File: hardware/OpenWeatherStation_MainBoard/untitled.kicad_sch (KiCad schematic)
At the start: 46 parts, among them Q1 Q_NMOS_GDS, U5 PM8800A, U6 POE13P-33L

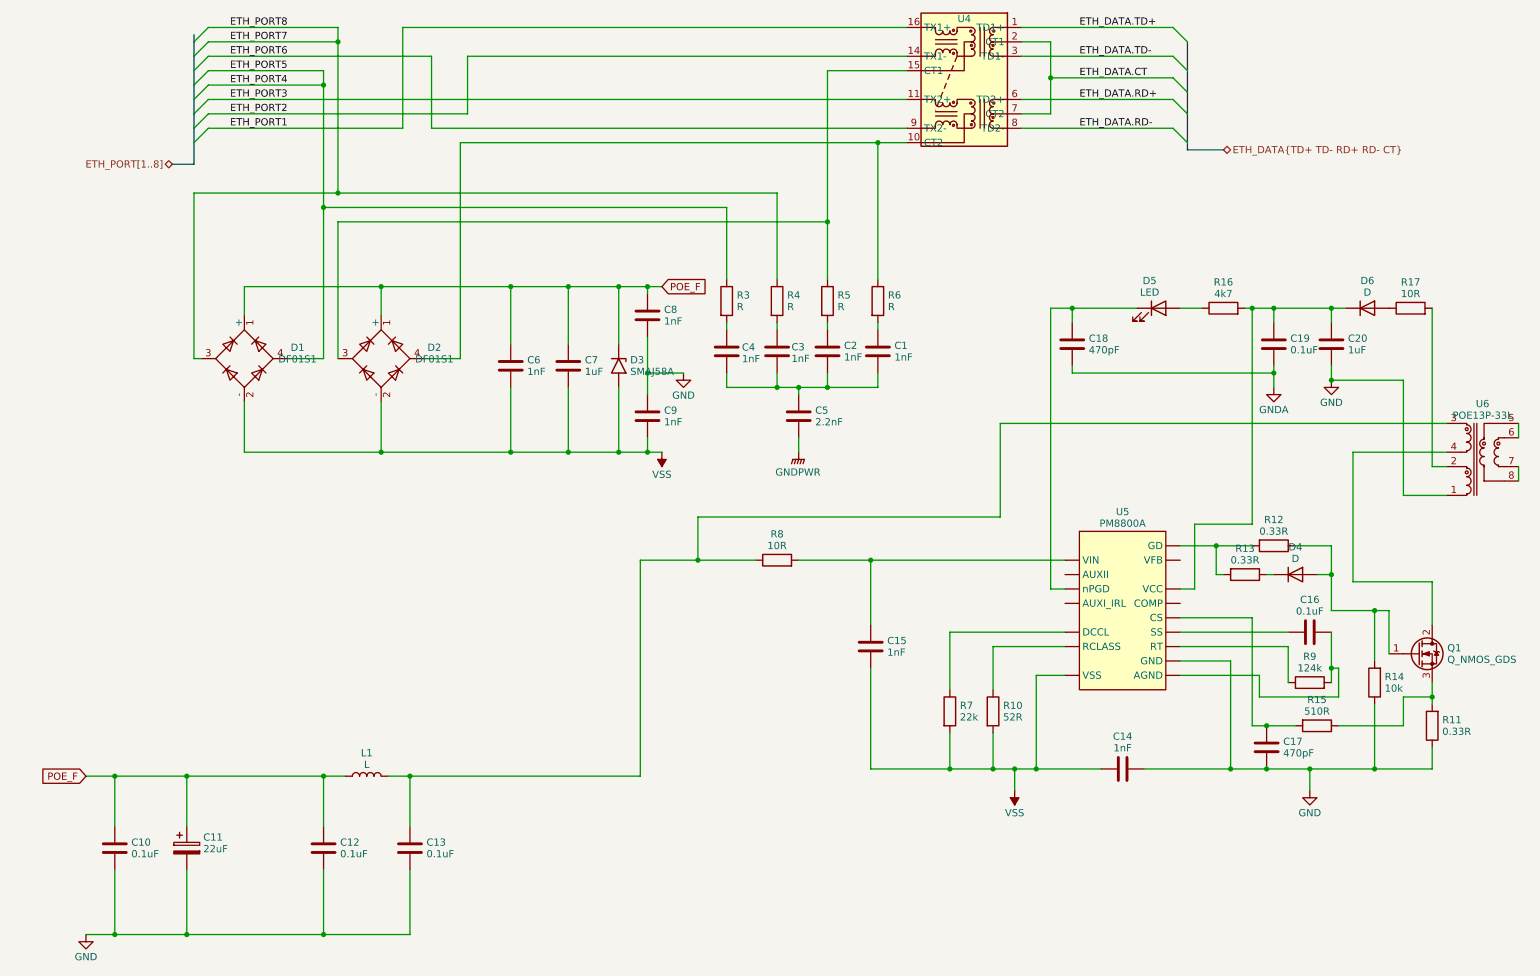
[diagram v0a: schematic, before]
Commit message: poe wip
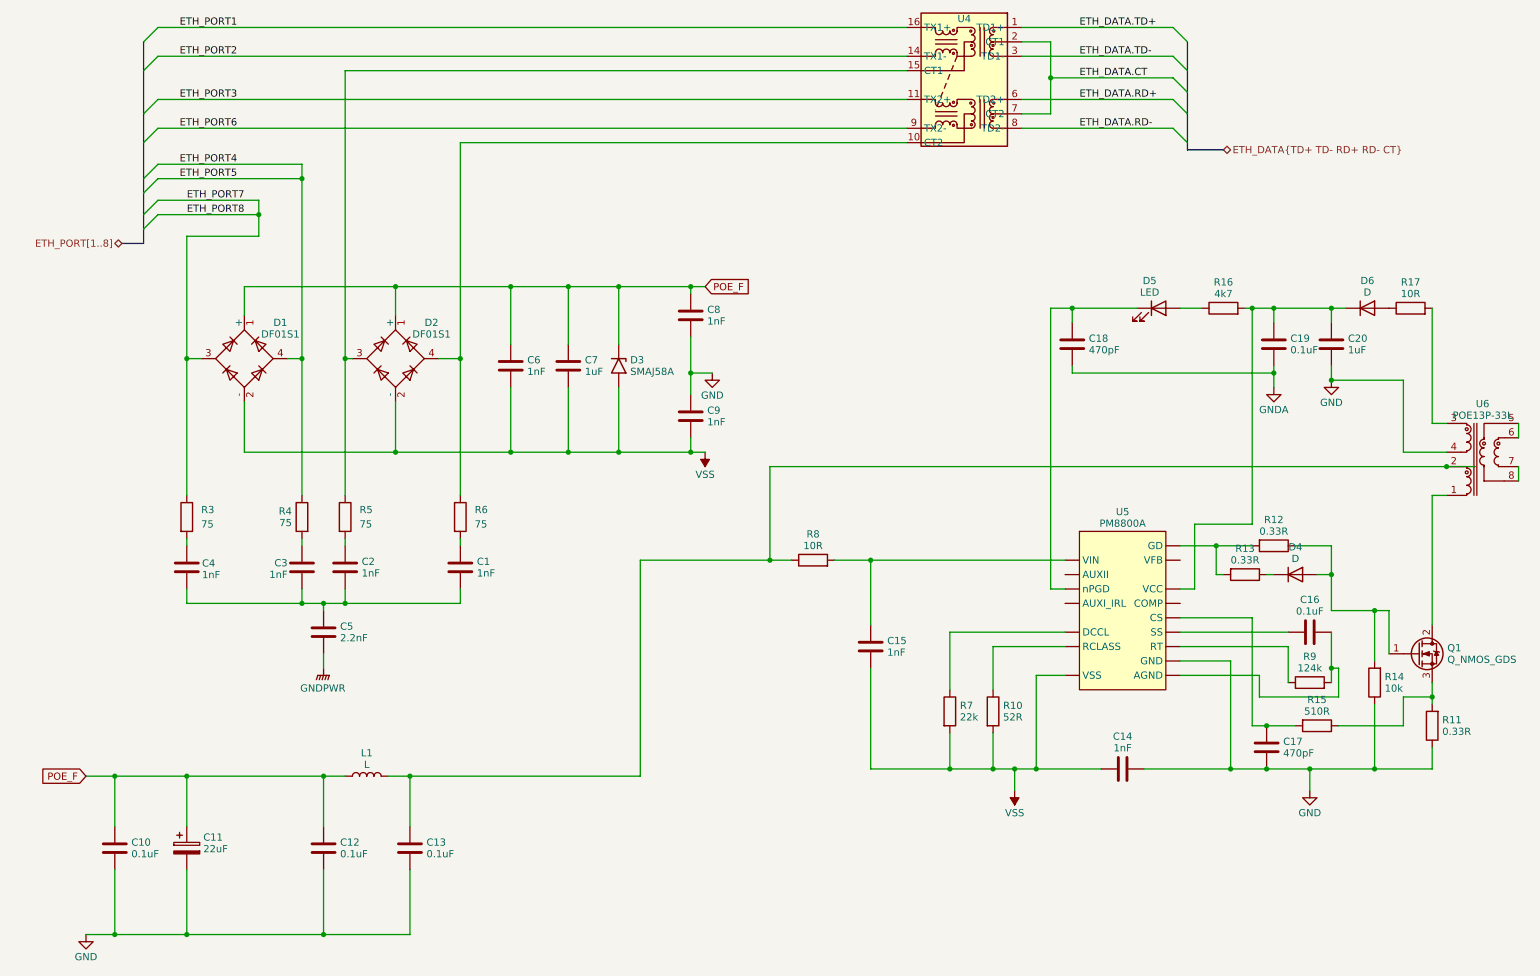
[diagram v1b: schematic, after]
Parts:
- R3, R4, R5, R6: value R -> 75
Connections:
- net ETH_PORT4: now also R4.1; no longer R3.1
- net ETH_PORT7: now also R3.1; no longer R4.1
- net GND: now also U6.4; no longer U6.1
- net at C13.1, L1.2, R8.1: now also U6.2; no longer U6.3
- net at Q1.2 (D): now also U6.1; no longer U6.4
- net at R17.2: now also U6.3; no longer U6.2
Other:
- moved on the sheet: C1, C2, C3, C4, C5, C8, C9, D2, R3, R4, R5, R6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
